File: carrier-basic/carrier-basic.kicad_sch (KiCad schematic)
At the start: 11 parts, among them J1 Conn_02x20_Counter_Clockwise, J2 Conn_02x20_Counter_Clockwise, J3 Conn_02x20_Counter_Clockwise, J4 Conn_02x20_Counter_Clockwise, J5 Conn_02x20_Counter_Clockwise, J6 Conn_02x20_Counter_Clockwise, J7 Conn_02x20_Counter_Clockwise

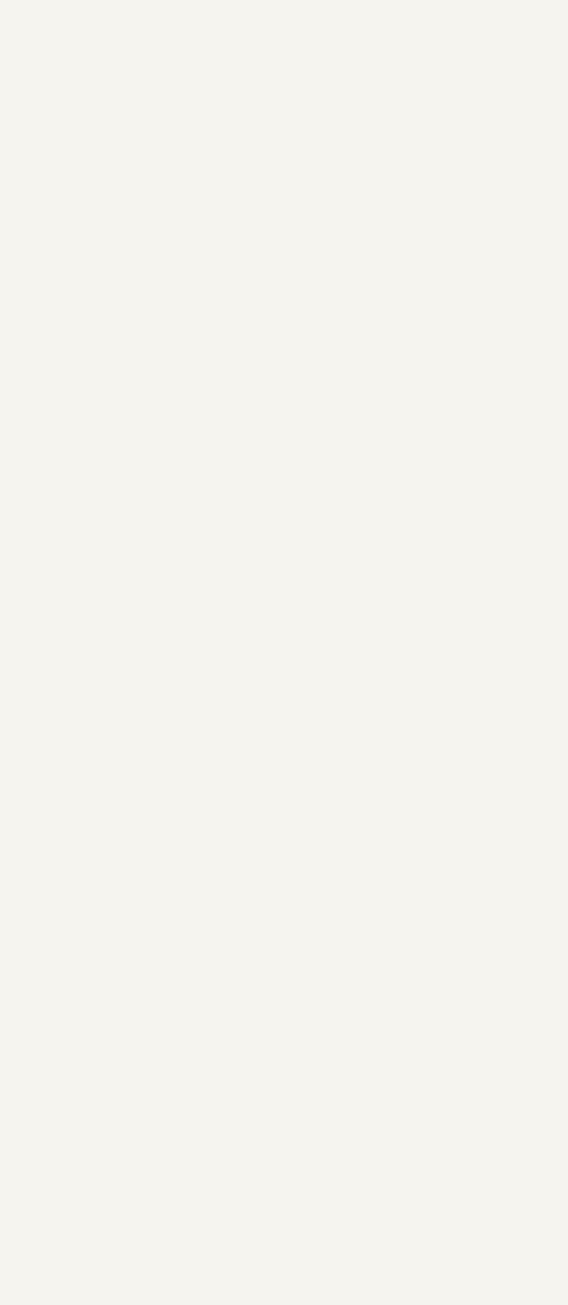
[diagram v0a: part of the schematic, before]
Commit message: Experiment with how I want to place some I/O on the basic carrier
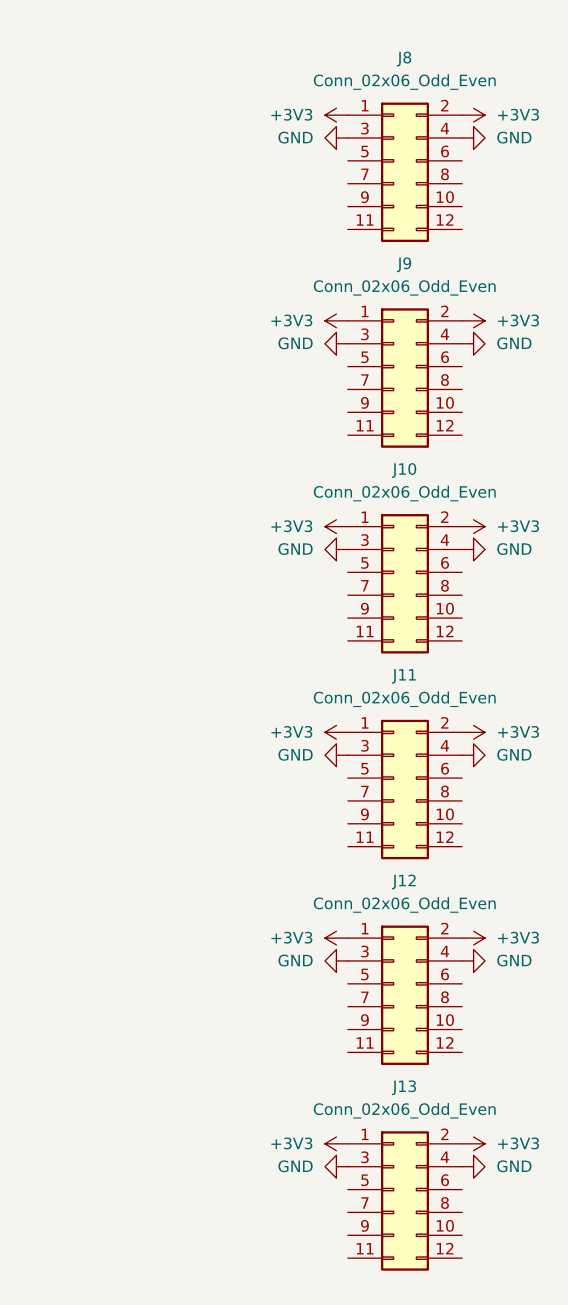
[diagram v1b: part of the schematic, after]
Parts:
- added J10, J11, J12, J13, J8, J9: Conn_02x06_Odd_Even, Connector_PinSocket_2.54mm:PinSocket_2x06_P2.54mm_Horizontal, symbol Connector_Generic:Conn_02x06_Odd_Even
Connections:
- net +3V3: now also J10.1 (Pin_1), J10.2 (Pin_2), J11.1 (Pin_1), J11.2 (Pin_2), J12.1 (Pin_1), J12.2 (Pin_2), J13.1 (Pin_1), J13.2 (Pin_2), J8.1 (Pin_1), J8.2 (Pin_2), J9.1 (Pin_1), J9.2 (Pin_2)
- net GND: now also J10.3 (Pin_3), J10.4 (Pin_4), J11.3 (Pin_3), J11.4 (Pin_4), J12.3 (Pin_3), J12.4 (Pin_4), J13.3 (Pin_3), J13.4 (Pin_4), J8.3 (Pin_3), J8.4 (Pin_4), J9.3 (Pin_3), J9.4 (Pin_4)
